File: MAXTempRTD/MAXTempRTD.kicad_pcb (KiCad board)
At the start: 2 copper layers, 26.2 x 29.2 mm, 24 parts, among them P1 RTD1, P2 RTD2, P3 OUTPUT, P4 INPUT, U1 MAX31865, U2 MAX31865

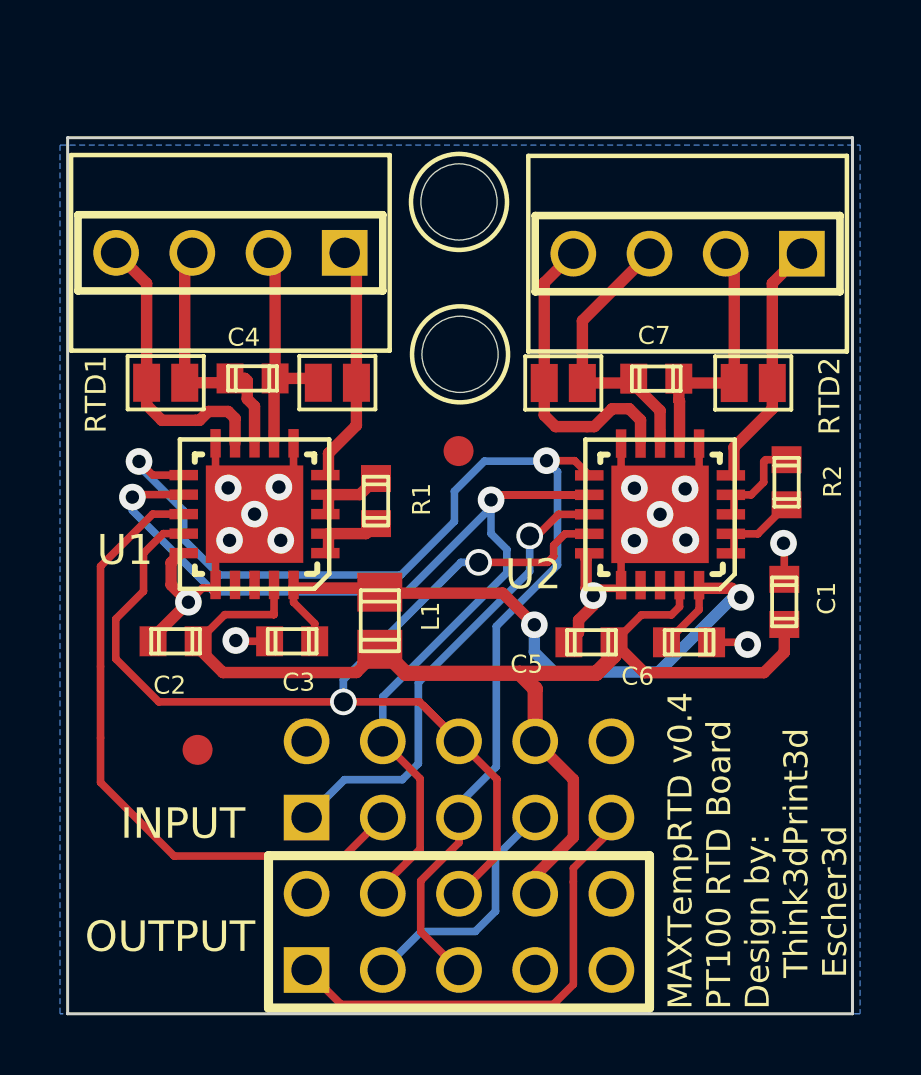
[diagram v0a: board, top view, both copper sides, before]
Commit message: Updated v1.1 source files
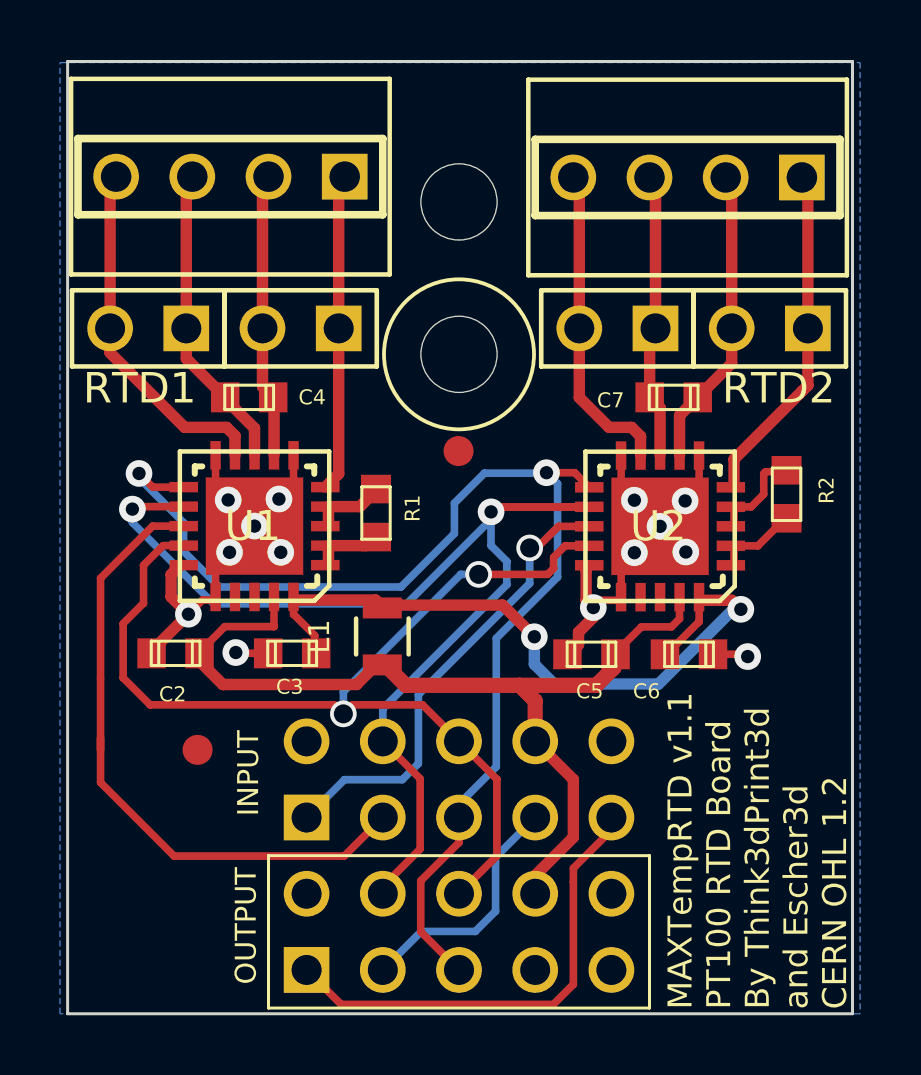
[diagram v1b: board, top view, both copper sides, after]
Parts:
- removed C1: 0.1u, c_0603
- removed Mount (x2): VAL**, Mount
- removed SJ1, SJ2, SJ3, SJ4: SJ, complib:SJ
- added G***: LOGO, complib:LOGO_Duet3dCompatible_xs, B.Cu at (62.9, 54.4)
- added J1: J, complib:JUMPER, F.Cu at (67.4, 36.3)
- added J2: J, complib:JUMPER, F.Cu at (62.3, 36.3)
- added J3: J, complib:JUMPER, F.Cu at (83.0, 36.3)
- added J4: J, complib:JUMPER, F.Cu at (77.9, 36.3)
- C2, C3, C4, C5, C6, C7: footprint c_0603 -> complib:C_0603
- L1: footprint c_0805 -> complib:R_0805
- P1, P2: footprint SCREW_TERMINAL_4x1 -> complib:SCREW_TERMINAL_4x1
- P3: footprint PIN_ARRAY_5x2 -> complib:MAX_TEMP_DB
- P4: footprint PIN_ARRAY_5x2 -> complib:MAX_TEMP_DB_inv; moved to B.Cu
- R1, R2: footprint c_0603 -> complib:R_0603
- U1, U2: footprint QFN20_5x5 -> complib:QFN20_5x5
- moved P1 2.54 mm to (65.0, 31.2)
- moved P2 2.54 mm to (80.3, 31.3)
- moved C7 0.85 mm to (79.8, 38.6)
- moved C4 0.64 mm to (65.7, 38.6)
- moved L1 0.53 mm to (70.1, 46.6), turned to 90 degrees
- moved C2 0.40 mm to (63.2, 47.1)
- moved C3 0.40 mm to (67.1, 47.1)
- moved R1 0.40 mm to (69.9, 42.5)
- moved C5 0.40 mm to (77.1, 47.2)
- moved C6 0.40 mm to (80.3, 47.2)
- moved R2 0.40 mm to (83.6, 41.8)
- moved U1 0.40 mm to (65.8, 42.9)
- moved U2 0.40 mm to (79.3, 42.9)
- turned P4 to 180 degrees
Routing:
- net 3.3V: track 39.9 -> 32.6 mm
- net RC_2_A1: track 8.33 -> 11.4 mm
- net RC_1_A1: track 7.96 -> 10.6 mm
- net RC_1_B2: track 9.70 -> 11.9 mm
- net RC_1_A2: track 7.85 -> 9.72 mm
- net MISO: track 37.1 -> 35.3 mm
- net RC_2_A2: track 8.40 -> 10.1 mm
- net RC_1_B1: track 8.69 -> 10.2 mm
- net GND: track 50.7 -> 49.5 mm, vias 15 -> 14
- net Net-(R2-Pad2): track 3.29 -> 2.58 mm
- net Net-(R2-Pad1): track 2.81 -> 3.51 mm
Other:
- board size 26.2 x 29.2 mm -> 26.2 x 31.7 mm
- board text added: "MAXTempRTD v1.1 PT100 RTD Board By Think3dPrint3d and Escher3d CERN OHL 1.2"
- board text removed: "MAXTempRTD v0.4 PT100 RTD Board Design by: Think3dPrint3d Escher3d"
